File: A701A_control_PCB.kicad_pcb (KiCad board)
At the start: 2 copper layers, 10 parts, among them P1 CONN_2, P2 CONN_2

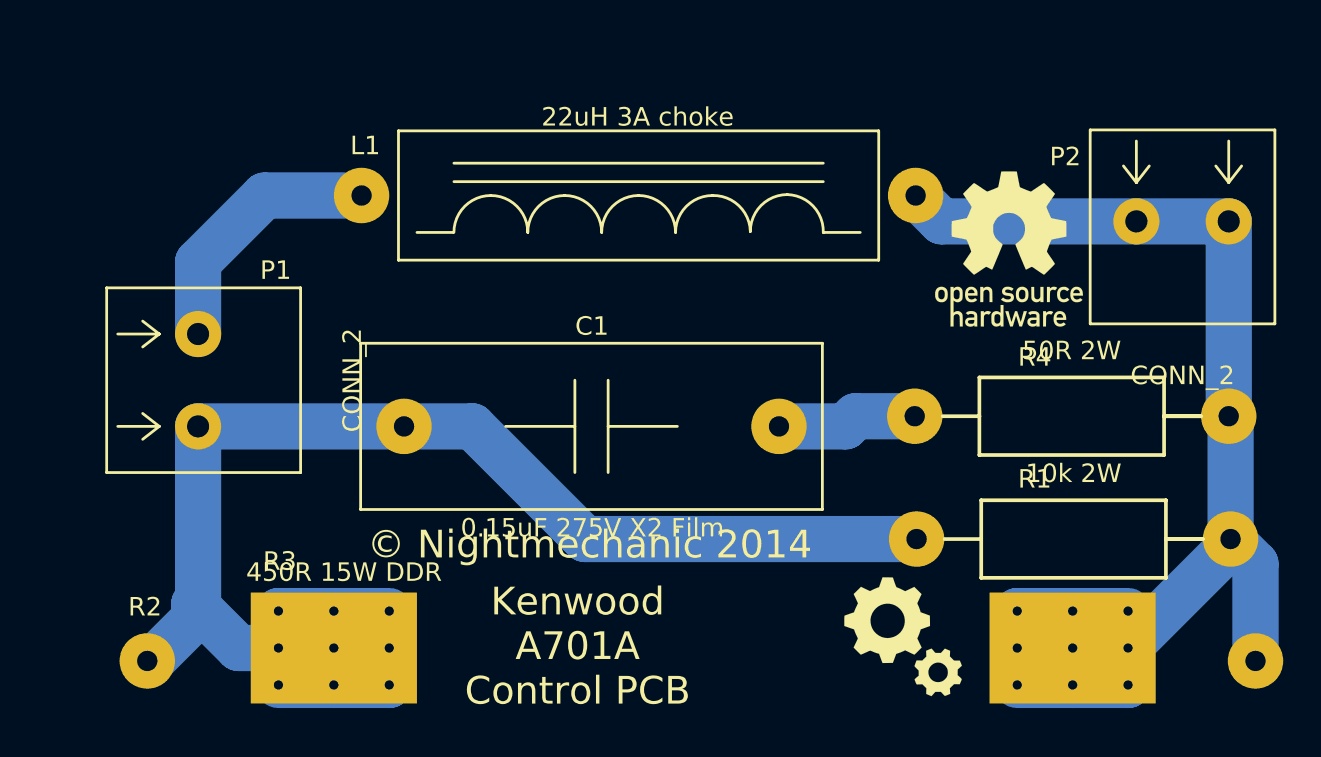
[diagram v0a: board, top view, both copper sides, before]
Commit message: Layout done
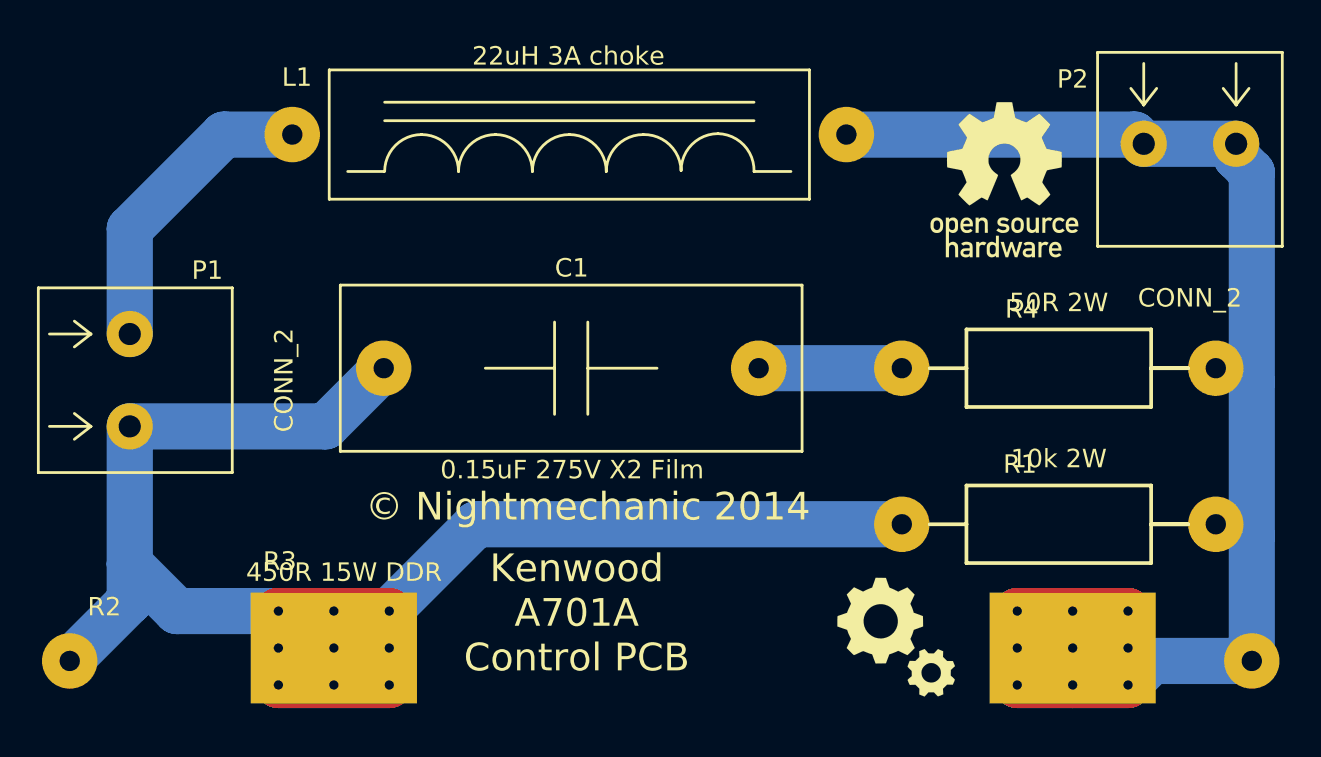
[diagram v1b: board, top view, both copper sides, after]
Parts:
- moved L1 5.00 mm to (92.8, 32.2)
- moved P2 4.22 mm to (126.3, 32.7)
- moved VAL 3.76 mm to (116.3, 34.6)
- moved P1 3.70 mm to (69.0, 45.5)
- moved C1 3.34 mm to (92.8, 44.9)
- moved R4 2.69 mm to (119.2, 44.9)
- moved R2 2.20 mm to (97.7, 60.7)
- moved R1 1.13 mm to (119.2, 53.3)
- moved VAL 0.38 mm to (110.5, 59.4)
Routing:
- net Net-(C1-Pad1): track 83.0 -> 146.9 mm
- net Net-(L1-Pad2): track 72.1 -> 132.4 mm
- net Net-(L1-Pad1): track 14.2 -> 16.6 mm
